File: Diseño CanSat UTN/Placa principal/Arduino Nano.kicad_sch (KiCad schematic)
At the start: 3 parts, among them J2 Conn_01x15_MountingPin, J3 Conn_01x15_MountingPin

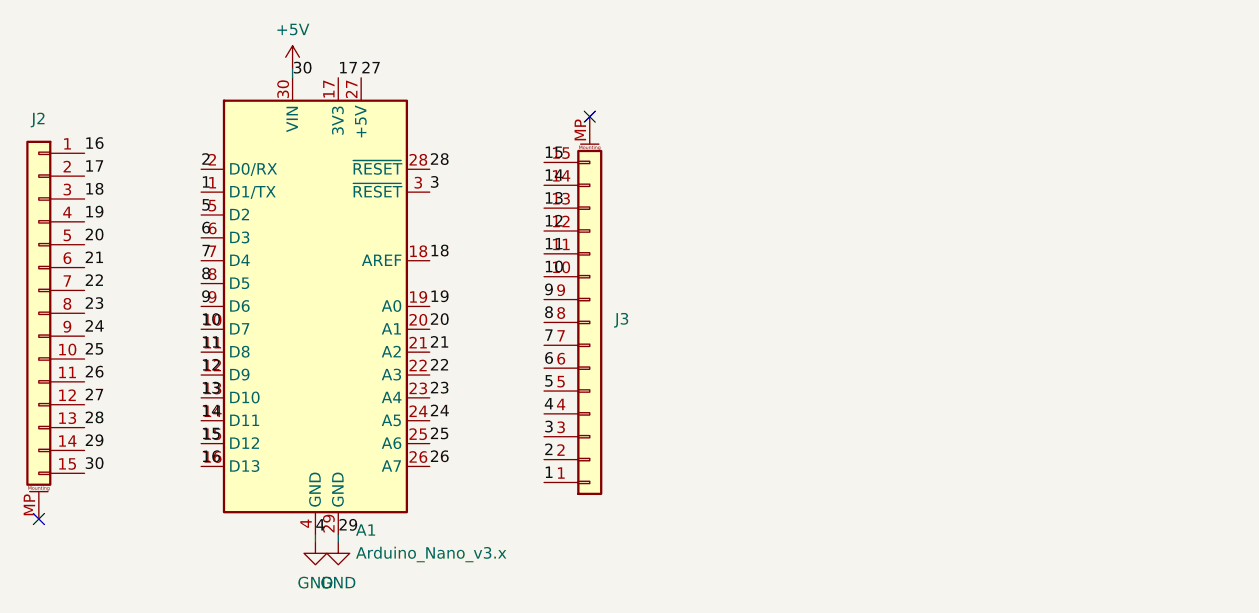
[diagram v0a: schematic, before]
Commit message: Actualizando diseño
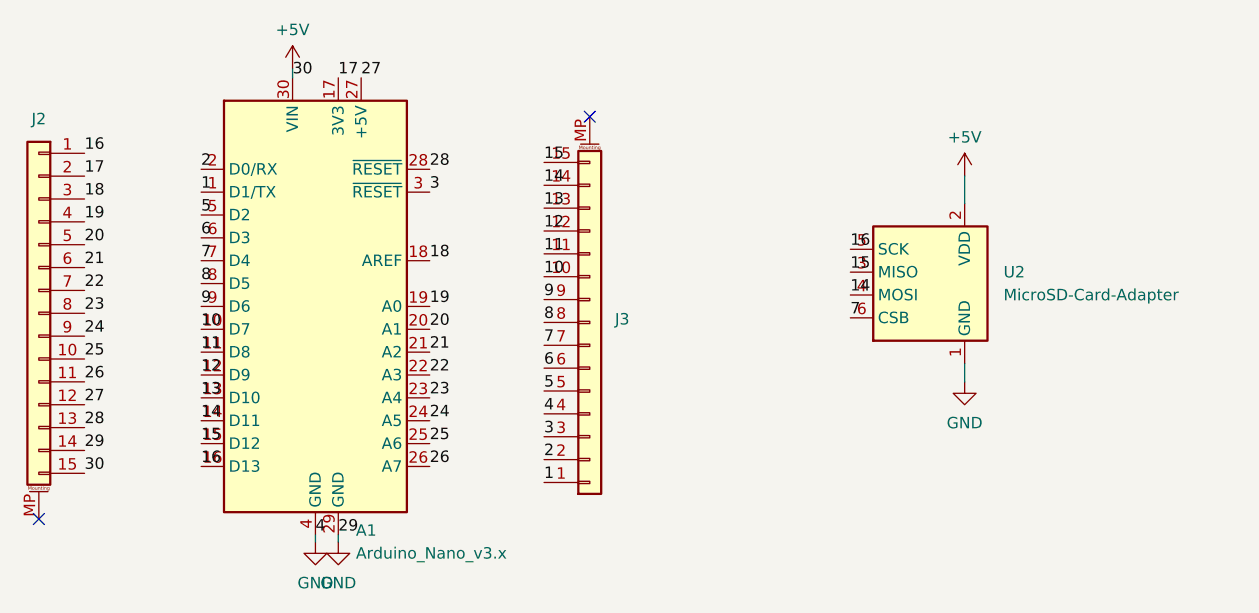
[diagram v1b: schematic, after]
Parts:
- added U2: MicroSD-Card-Adapter, MicroSD-Card-Adapter:MicroSD-Card-Adapter, symbol Sensor_Pressure:BMP280
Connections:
- net +5V: now also U2.2 (VDD)
- net 14: now also U2.4 (MOSI)
- net 15: now also U2.3 (MISO)
- net 16: now also U2.5 (SCK)
- net 7: now also U2.6 (CSB)
- net GND: now also U2.1 (GND)
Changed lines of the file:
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@@
     (stroke (width 0) (type default))
   )
+  (wire (pts (xy 169.164 49.53) (xy 169.164 52.578))
+    (stroke (width 0) (type default))
+  )
+  (wire (pts (xy 169.164 72.39) (xy 169.164 70.358))
+    (stroke (width 0) (type default))
+  )
   (label "17" (at 99.568 38.608 0) (fields_autoplaced)
     (effects (font (size 1.27 1.27)) (justify left bottom))
@@
     (effects (font (size 1.27 1.27)) (justify left bottom))
   )
+  (label "14" (at 156.464 62.738 0) (fields_autoplaced)
+    (effects (font (size 1.27 1.27)) (justify left bottom))
+  )
   (label "12" (at 84.328 71.628 0) (fields_autoplaced)
     (effects (font (size 1.27 1.27)) (justify left bottom))
@@
     (effects (font (size 1.27 1.27)) (justify left bottom))
   )
+  (label "15" (at 156.464 60.198 0) (fields_autoplaced)
+    (effects (font (size 1.27 1.27)) (justify left bottom))
+  )
   (label "27" (at 71.374 74.93 0) (fields_autoplaced)
     (effects (font (size 1.27 1.27)) (justify left bottom))
@@
     (effects (font (size 1.27 1.27)) (justify left bottom))
   )
+  (label "16" (at 156.464 57.658 0) (fields_autoplaced)
+    (effects (font (size 1.27 1.27)) (justify left bottom))
+  )
   (label "15" (at 122.428 48.006 0) (fields_autoplaced)
     (effects (font (size 1.27 1.27)) (justify left bottom))
@@
     (effects (font (size 1.27 1.27)) (justify left bottom))
   )
+  (label "7" (at 156.464 65.278 0) (fields_autoplaced)
+    (effects (font (size 1.27 1.27)) (justify left bottom))
+  )
   (label "27" (at 102.108 38.608 0) (fields_autoplaced)
     (effects (font (size 1.27 1.27)) (justify left bottom))
@@
   (label "8" (at 84.328 61.468 0) (fields_autoplaced)
     (effects (font (size 1.27 1.27)) (justify left bottom))
+  )
+  (symbol (lib_id "Sensor_Pressure:BMP280") (at 166.624 62.738 0) (unit 1)
+    (in_bom yes) (on_board yes) (dnp no) (fields_autoplaced)
+    (property "Reference" "U2" (at 173.482 60.198 0)
+      (effects (font (size 1.27 1.27)) (justify left))
+    )
+    (property "Value" "MicroSD-Card-Adapter" (at 173.482 62.738 0)
+      (effects (font (size 1.27 1.27)) (justify left))
+    )
+    (property "Footprint" "MicroSD-Card-Adapter:MicroSD-Card-Adapter" (at 166.624 80.518 0)
+      (effects (font (size 1.27 1.27)) hide)
+    )
+    (property "Datasheet" "https://ae-bst.resource.bosch.com/media/_tech/media/datasheets/BST-BMP280-DS001.pdf" (at 166.624 76.708 0)
+      (effects (font (size 1.27 1.27)) hide)
+    )
+    (pin "1")
+    (pin "2")
+    (pin "3")
+    (pin "4")
+    (pin "5")
+    (pin "6")
+    (instances
+      (project "Diseño CanSat UTN"
+        (path "/6d01f5e8-1e9f-449b-95d5-6b60605ac758/7a421331-9374-4963-972d-5d2825b48499"
+          (reference "U2") (unit 1)
+        )
+      )
+    )
+  )
+  (symbol (lib_id "power:+5V") (at 169.164 49.53 0) (unit 1)
+    (in_bom yes) (on_board yes) (dnp no) (fields_autoplaced)
+    (property "Reference" "#PWR014" (at 169.164 53.34 0)
+      (effects (font (size 1.27 1.27)) hide)
+    )
+    (property "Value" "+5V" (at 169.164 45.212 0)
+      (effects (font (size 1.27 1.27)))
+    )
+    (property "Footprint" "" (at 169.164 49.53 0)
+      (effects (font (size 1.27 1.27)) hide)
+    )
+    (property "Datasheet" "" (at 169.164 49.53 0)
+      (effects (font (size 1.27 1.27)) hide)
+    )
+    (pin "1")
+    (instances
+      (project "Diseño CanSat UTN"
+        (path "/6d01f5e8-1e9f-449b-95d5-6b60605ac758/7a421331-9374-4963-972d-5d2825b48499"
+          (reference "#PWR014") (unit 1)
+        )
+      )
+    )
   )
   (symbol (lib_id "Connector_Generic_MountingPin:Conn_01x15_MountingPin") (at 66.294 64.77 0) (mirror y) (unit 1)
@@
         )
       )
+    )
+  )
+  (symbol (lib_id "power:GND") (at 169.164 72.39 0) (unit 1)
+    (in_bom yes) (on_board yes) (dnp no) (fields_autoplaced)
+    (property "Reference" "#PWR013" (at 169.164 78.74 0)
+      (effects (font (size 1.27 1.27)) hide)
+    )
+    (property "Value" "GND" (at 169.164 76.962 0)
+      (effects (font (size 1.27 1.27)))
+    )
+    (property "Footprint" "" (at 169.164 72.39 0)
+      (effects (font (size 1.27 1.27)) hide)
+    )
+    (property "Datasheet" "" (at 169.164 72.39 0)
+      (effects (font (size 1.27 1.27)) hide)
+    )
+    (pin "1")
+    (instances
+      (project "Diseño CanSat UTN"
+        (path "/6d01f5e8-1e9f-449b-95d5-6b60605ac758/7a421331-9374-4963-972d-5d2825b48499"
+          (reference "#PWR013") (unit 1)
+        )
+      )
